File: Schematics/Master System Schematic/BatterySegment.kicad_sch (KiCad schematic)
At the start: 148 parts

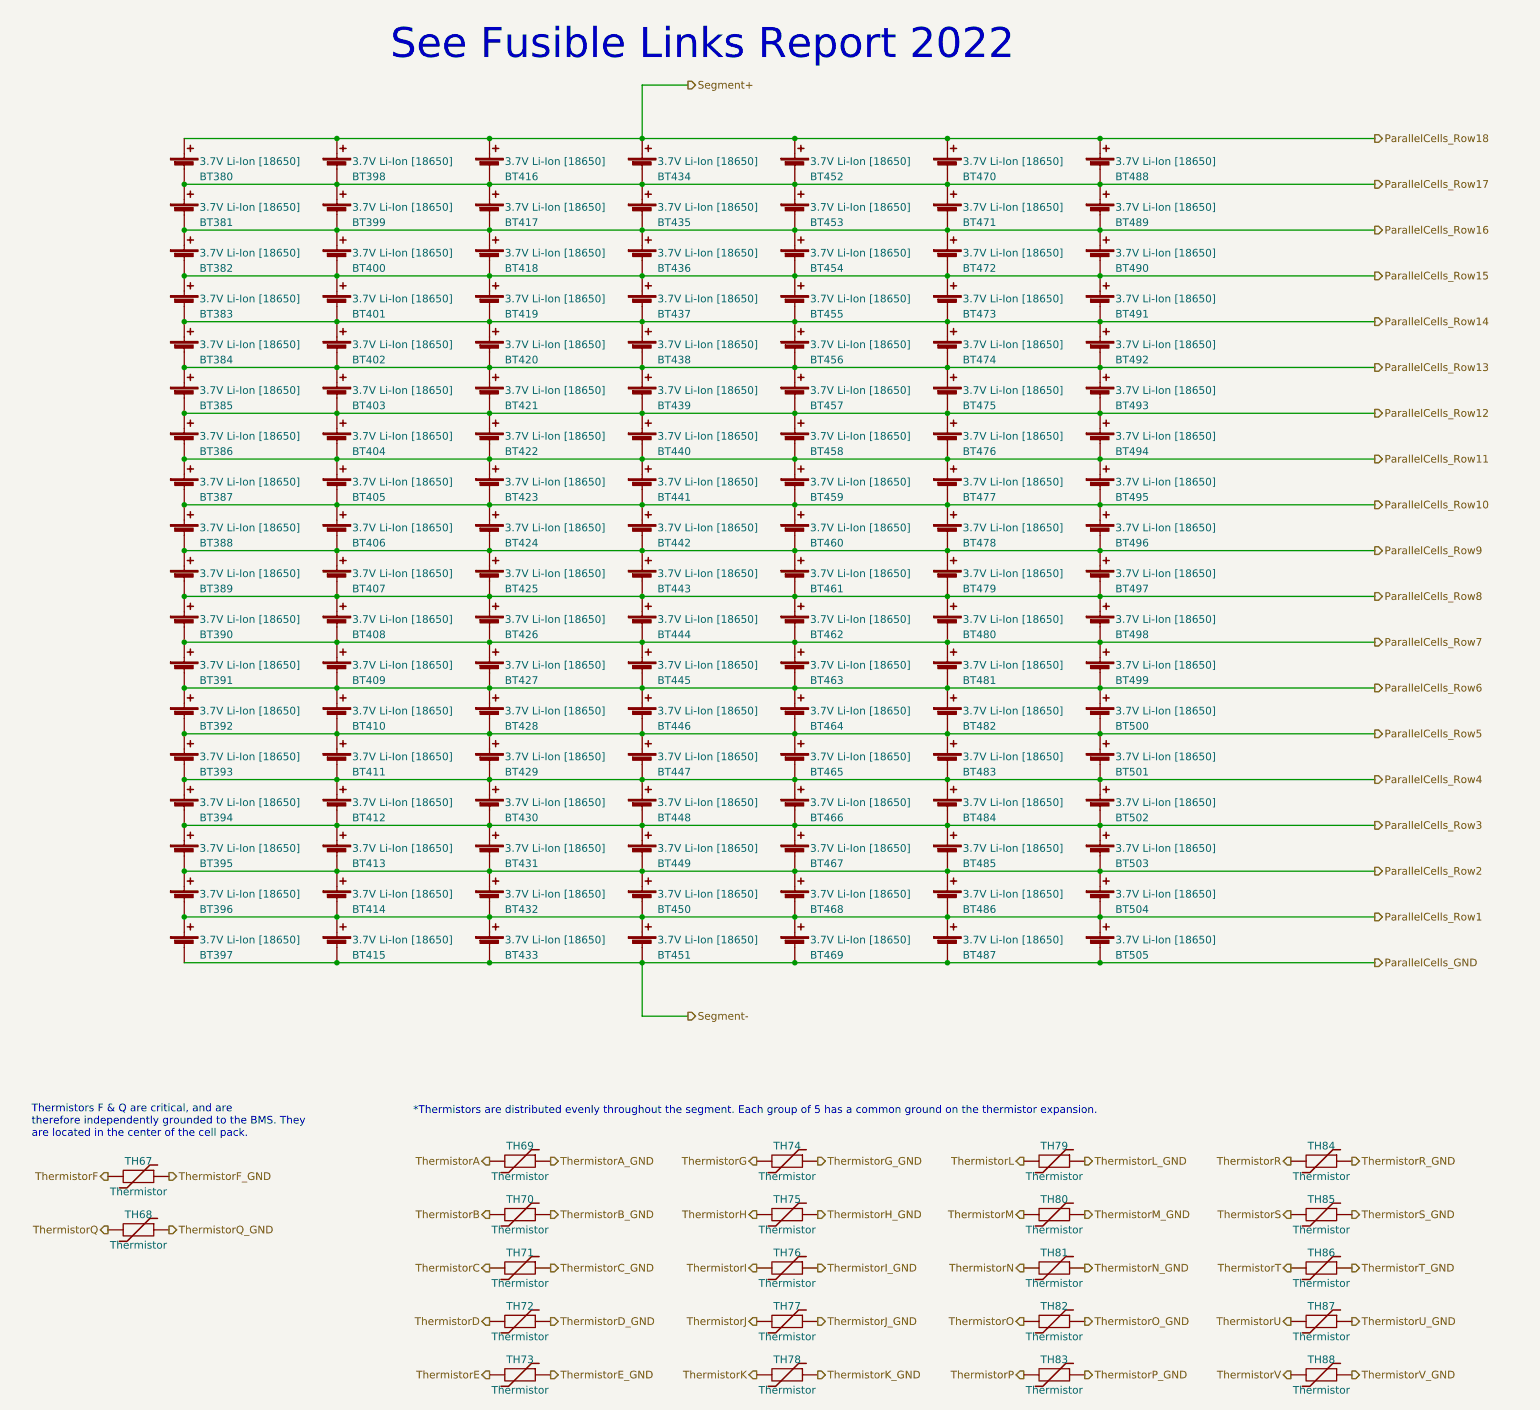
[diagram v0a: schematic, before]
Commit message: ESF-2 2023 Updates (#136)
* Moved shutdown loop & TSMPs

* Moved Dashboard/Footwellbox

* Deleted SSOKs

* More stuff

* Charger and battbox stuff

* Added battbox fans

* Updated sheet sizing

* Flipped MC

 to make powertrain ordering better

* Updated HV plate

* IDrk

* Better topsheet labels

* Segment Layer updates

Adding shepherd

* LV Plate update

* Partial work on accumulator container sheet

To be continued

* Finish accumulator

* Footwell updates

* Removing old files

* Added Wheel

* Top sheet budge

* Renumbered pages

* Shutdown Summary Updates

* Missed some TSV color

* Export shutdown summary

* Deleted more old files

* Added TSAL17

* Added TS-GLV17

* Added Wheel17

* Other NER lib cleanup

* Annotations

* More annotate and export

* Moved PDF

* Reexport master schem

* Cleaning out old shutdown summary files

* MATLAB!

For precharge and discharge plotting

* Changed label alignment

* Updated dashboard name

* Updated for LFP board and bigger top sheet

* backup

* Changed breaker to fuse in Shutdown Simmary

* Finished traces

* Oops forgot to merge
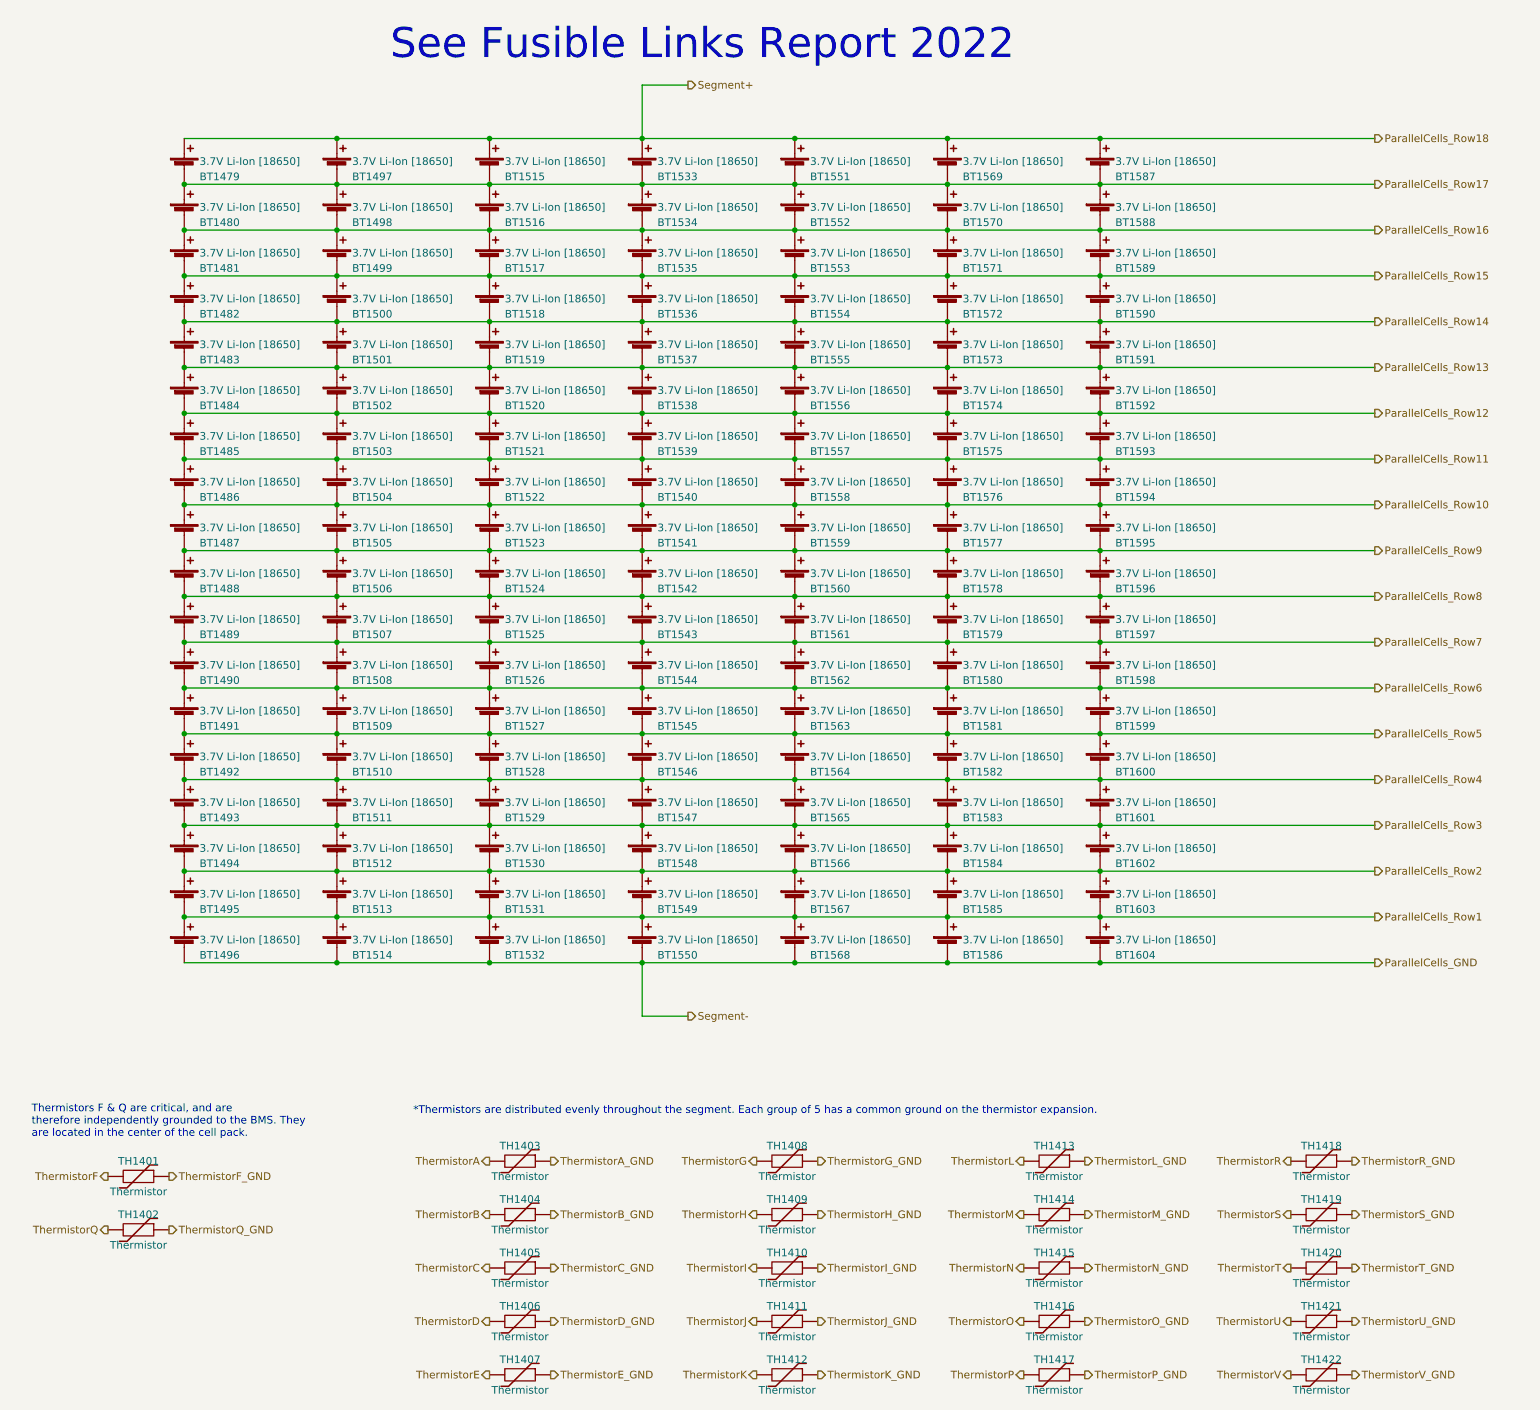
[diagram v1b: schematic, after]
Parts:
- renumbered BT380 to BT1479, BT381 to BT1480, BT382 to BT1481, BT383 to BT1482, BT384 to BT1483, BT385 to BT1484, BT386 to BT1485, BT387 to BT1486, BT388 to BT1487, BT389 to BT1488, BT390 to BT1489, BT391 to BT1490, BT392 to BT1491, BT393 to BT1492, BT394 to BT1493, BT395 to BT1494, BT396 to BT1495, BT397 to BT1496, BT398 to BT1497, BT399 to BT1498, BT400 to BT1499, BT401 to BT1500, BT402 to BT1501, BT403 to BT1502, BT404 to BT1503, BT405 to BT1504, BT406 to BT1505, BT407 to BT1506, BT408 to BT1507, BT409 to BT1508, BT410 to BT1509, BT411 to BT1510, BT412 to BT1511, BT413 to BT1512, BT414 to BT1513, BT415 to BT1514, BT416 to BT1515, BT417 to BT1516, BT418 to BT1517, BT419 to BT1518, BT420 to BT1519, BT421 to BT1520, BT422 to BT1521, BT423 to BT1522, BT424 to BT1523, BT425 to BT1524, BT426 to BT1525, BT427 to BT1526, BT428 to BT1527, BT429 to BT1528, BT430 to BT1529, BT431 to BT1530, BT432 to BT1531, BT433 to BT1532, BT434 to BT1533, BT435 to BT1534, BT436 to BT1535, BT437 to BT1536, BT438 to BT1537, BT439 to BT1538, BT440 to BT1539, BT441 to BT1540, BT442 to BT1541, BT443 to BT1542, BT444 to BT1543, BT445 to BT1544, BT446 to BT1545, BT447 to BT1546, BT448 to BT1547, BT449 to BT1548, BT450 to BT1549, BT451 to BT1550, BT452 to BT1551, BT453 to BT1552, BT454 to BT1553, BT455 to BT1554, BT456 to BT1555, BT457 to BT1556, BT458 to BT1557, BT459 to BT1558, BT460 to BT1559, BT461 to BT1560, BT462 to BT1561, BT463 to BT1562, BT464 to BT1563, BT465 to BT1564, BT466 to BT1565, BT467 to BT1566, BT468 to BT1567, BT469 to BT1568, BT470 to BT1569, BT471 to BT1570, BT472 to BT1571, BT473 to BT1572, BT474 to BT1573, BT475 to BT1574, BT476 to BT1575, BT477 to BT1576, BT478 to BT1577, BT479 to BT1578, BT480 to BT1579, BT481 to BT1580, BT482 to BT1581, BT483 to BT1582, BT484 to BT1583, BT485 to BT1584, BT486 to BT1585, BT487 to BT1586, BT488 to BT1587, BT489 to BT1588, BT490 to BT1589, BT491 to BT1590, BT492 to BT1591, BT493 to BT1592, BT494 to BT1593, BT495 to BT1594, BT496 to BT1595, BT497 to BT1596, BT498 to BT1597, BT499 to BT1598, BT500 to BT1599, BT501 to BT1600, BT502 to BT1601, BT503 to BT1602, BT504 to BT1603, BT505 to BT1604, TH67 to TH1401, TH68 to TH1402, TH69 to TH1403, TH70 to TH1404, TH71 to TH1405, TH72 to TH1406, TH73 to TH1407, TH74 to TH1408, TH75 to TH1409, TH76 to TH1410, TH77 to TH1411, TH78 to TH1412, TH79 to TH1413, TH80 to TH1414, TH81 to TH1415, TH82 to TH1416, TH83 to TH1417, TH84 to TH1418, TH85 to TH1419, TH86 to TH1420, TH87 to TH1421, TH88 to TH1422

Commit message: Revert "ESF-2 2023 Updates (#136)"
This reverts commit dbac7da28cdaad5f36fde89af32aad76a0b85ea3.
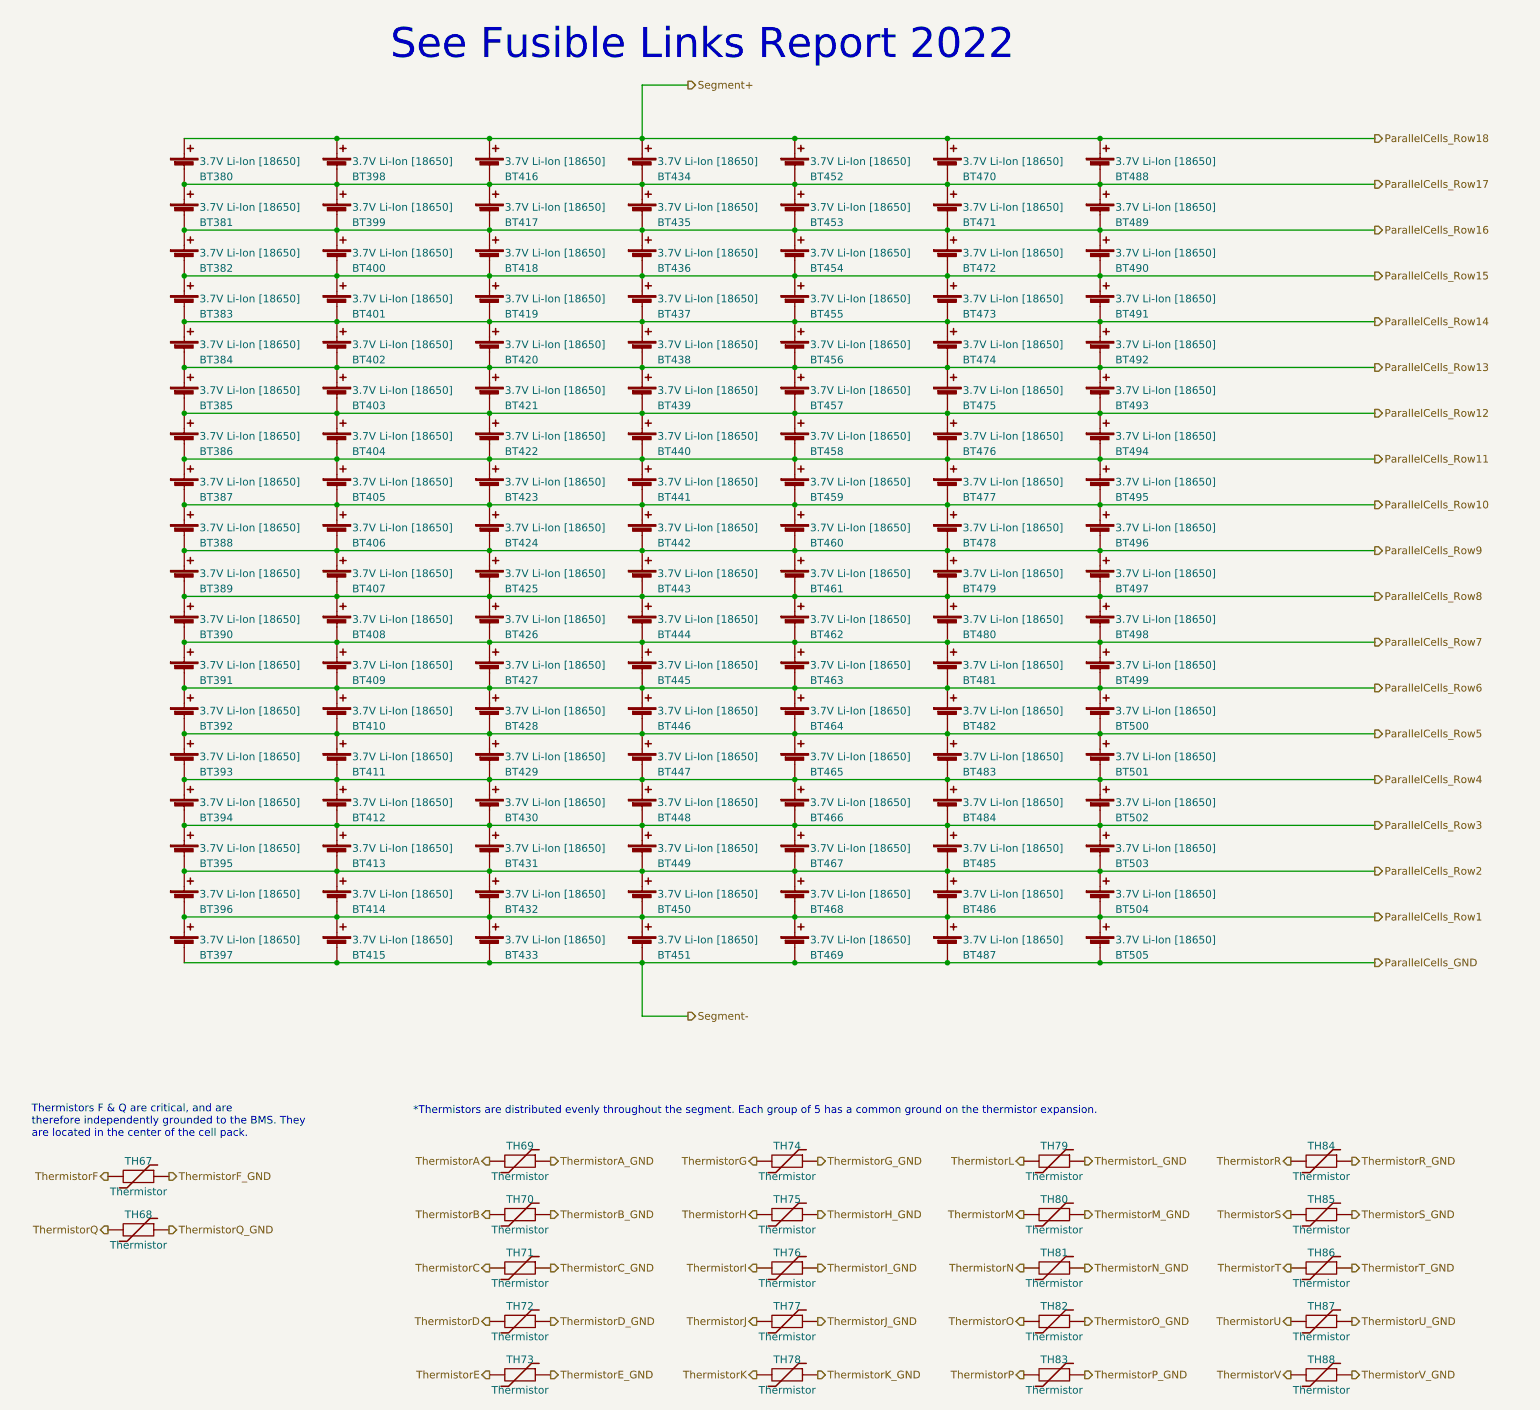
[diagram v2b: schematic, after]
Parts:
- renumbered BT1479 to BT380, BT1480 to BT381, BT1481 to BT382, BT1482 to BT383, BT1483 to BT384, BT1484 to BT385, BT1485 to BT386, BT1486 to BT387, BT1487 to BT388, BT1488 to BT389, BT1489 to BT390, BT1490 to BT391, BT1491 to BT392, BT1492 to BT393, BT1493 to BT394, BT1494 to BT395, BT1495 to BT396, BT1496 to BT397, BT1497 to BT398, BT1498 to BT399, BT1499 to BT400, BT1500 to BT401, BT1501 to BT402, BT1502 to BT403, BT1503 to BT404, BT1504 to BT405, BT1505 to BT406, BT1506 to BT407, BT1507 to BT408, BT1508 to BT409, BT1509 to BT410, BT1510 to BT411, BT1511 to BT412, BT1512 to BT413, BT1513 to BT414, BT1514 to BT415, BT1515 to BT416, BT1516 to BT417, BT1517 to BT418, BT1518 to BT419, BT1519 to BT420, BT1520 to BT421, BT1521 to BT422, BT1522 to BT423, BT1523 to BT424, BT1524 to BT425, BT1525 to BT426, BT1526 to BT427, BT1527 to BT428, BT1528 to BT429, BT1529 to BT430, BT1530 to BT431, BT1531 to BT432, BT1532 to BT433, BT1533 to BT434, BT1534 to BT435, BT1535 to BT436, BT1536 to BT437, BT1537 to BT438, BT1538 to BT439, BT1539 to BT440, BT1540 to BT441, BT1541 to BT442, BT1542 to BT443, BT1543 to BT444, BT1544 to BT445, BT1545 to BT446, BT1546 to BT447, BT1547 to BT448, BT1548 to BT449, BT1549 to BT450, BT1550 to BT451, BT1551 to BT452, BT1552 to BT453, BT1553 to BT454, BT1554 to BT455, BT1555 to BT456, BT1556 to BT457, BT1557 to BT458, BT1558 to BT459, BT1559 to BT460, BT1560 to BT461, BT1561 to BT462, BT1562 to BT463, BT1563 to BT464, BT1564 to BT465, BT1565 to BT466, BT1566 to BT467, BT1567 to BT468, BT1568 to BT469, BT1569 to BT470, BT1570 to BT471, BT1571 to BT472, BT1572 to BT473, BT1573 to BT474, BT1574 to BT475, BT1575 to BT476, BT1576 to BT477, BT1577 to BT478, BT1578 to BT479, BT1579 to BT480, BT1580 to BT481, BT1581 to BT482, BT1582 to BT483, BT1583 to BT484, BT1584 to BT485, BT1585 to BT486, BT1586 to BT487, BT1587 to BT488, BT1588 to BT489, BT1589 to BT490, BT1590 to BT491, BT1591 to BT492, BT1592 to BT493, BT1593 to BT494, BT1594 to BT495, BT1595 to BT496, BT1596 to BT497, BT1597 to BT498, BT1598 to BT499, BT1599 to BT500, BT1600 to BT501, BT1601 to BT502, BT1602 to BT503, BT1603 to BT504, BT1604 to BT505, TH1401 to TH67, TH1402 to TH68, TH1403 to TH69, TH1404 to TH70, TH1405 to TH71, TH1406 to TH72, TH1407 to TH73, TH1408 to TH74, TH1409 to TH75, TH1410 to TH76, TH1411 to TH77, TH1412 to TH78, TH1413 to TH79, TH1414 to TH80, TH1415 to TH81, TH1416 to TH82, TH1417 to TH83, TH1418 to TH84, TH1419 to TH85, TH1420 to TH86, TH1421 to TH87, TH1422 to TH88

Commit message: Moved shutdown loop & TSMPs
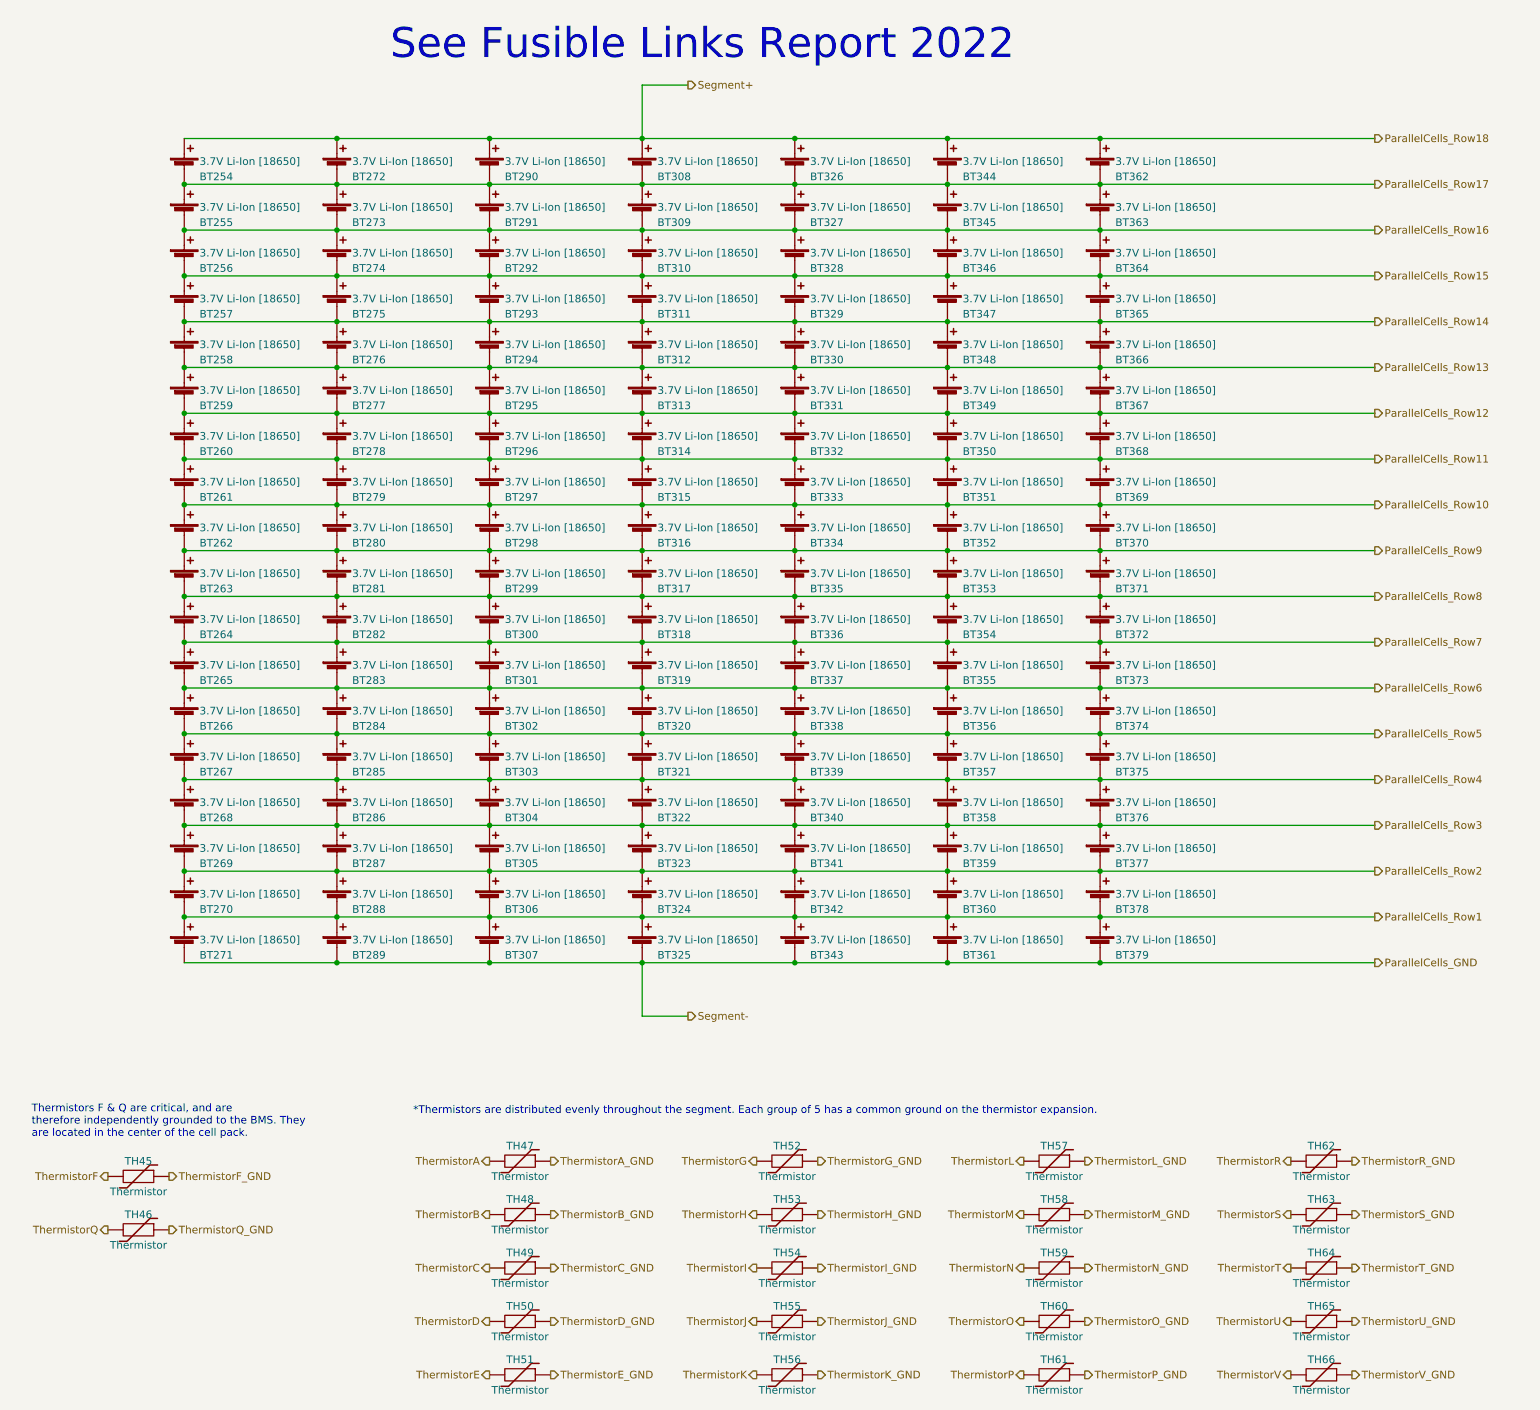
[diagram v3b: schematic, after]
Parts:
- renumbered BT380 to BT254, BT381 to BT255, BT382 to BT256, BT383 to BT257, BT384 to BT258, BT385 to BT259, BT386 to BT260, BT387 to BT261, BT388 to BT262, BT389 to BT263, BT390 to BT264, BT391 to BT265, BT392 to BT266, BT393 to BT267, BT394 to BT268, BT395 to BT269, BT396 to BT270, BT397 to BT271, BT398 to BT272, BT399 to BT273, BT400 to BT274, BT401 to BT275, BT402 to BT276, BT403 to BT277, BT404 to BT278, BT405 to BT279, BT406 to BT280, BT407 to BT281, BT408 to BT282, BT409 to BT283, BT410 to BT284, BT411 to BT285, BT412 to BT286, BT413 to BT287, BT414 to BT288, BT415 to BT289, BT416 to BT290, BT417 to BT291, BT418 to BT292, BT419 to BT293, BT420 to BT294, BT421 to BT295, BT422 to BT296, BT423 to BT297, BT424 to BT298, BT425 to BT299, BT426 to BT300, BT427 to BT301, BT428 to BT302, BT429 to BT303, BT430 to BT304, BT431 to BT305, BT432 to BT306, BT433 to BT307, BT434 to BT308, BT435 to BT309, BT436 to BT310, BT437 to BT311, BT438 to BT312, BT439 to BT313, BT440 to BT314, BT441 to BT315, BT442 to BT316, BT443 to BT317, BT444 to BT318, BT445 to BT319, BT446 to BT320, BT447 to BT321, BT448 to BT322, BT449 to BT323, BT450 to BT324, BT451 to BT325, BT452 to BT326, BT453 to BT327, BT454 to BT328, BT455 to BT329, BT456 to BT330, BT457 to BT331, BT458 to BT332, BT459 to BT333, BT460 to BT334, BT461 to BT335, BT462 to BT336, BT463 to BT337, BT464 to BT338, BT465 to BT339, BT466 to BT340, BT467 to BT341, BT468 to BT342, BT469 to BT343, BT470 to BT344, BT471 to BT345, BT472 to BT346, BT473 to BT347, BT474 to BT348, BT475 to BT349, BT476 to BT350, BT477 to BT351, BT478 to BT352, BT479 to BT353, BT480 to BT354, BT481 to BT355, BT482 to BT356, BT483 to BT357, BT484 to BT358, BT485 to BT359, BT486 to BT360, BT487 to BT361, BT488 to BT362, BT489 to BT363, BT490 to BT364, BT491 to BT365, BT492 to BT366, BT493 to BT367, BT494 to BT368, BT495 to BT369, BT496 to BT370, BT497 to BT371, BT498 to BT372, BT499 to BT373, BT500 to BT374, BT501 to BT375, BT502 to BT376, BT503 to BT377, BT504 to BT378, BT505 to BT379, TH67 to TH45, TH68 to TH46, TH69 to TH47, TH70 to TH48, TH71 to TH49, TH72 to TH50, TH73 to TH51, TH74 to TH52, TH75 to TH53, TH76 to TH54, TH77 to TH55, TH78 to TH56, TH79 to TH57, TH80 to TH58, TH81 to TH59, TH82 to TH60, TH83 to TH61, TH84 to TH62, TH85 to TH63, TH86 to TH64, TH87 to TH65, TH88 to TH66
